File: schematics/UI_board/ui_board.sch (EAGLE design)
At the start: 116 parts, among them IC10 74HCT32N, IC11 74HCT14N, IC12 74HCT14N, IC13 74HCT393N, IC2 74HCT151N, IC3 74HCT32N, IC4 74HCT74N, IC5 74HCT08N, IC6 74HCT32N, IC7 74HCT14N, IC8 74HCT373N, IC9 74HCT32N

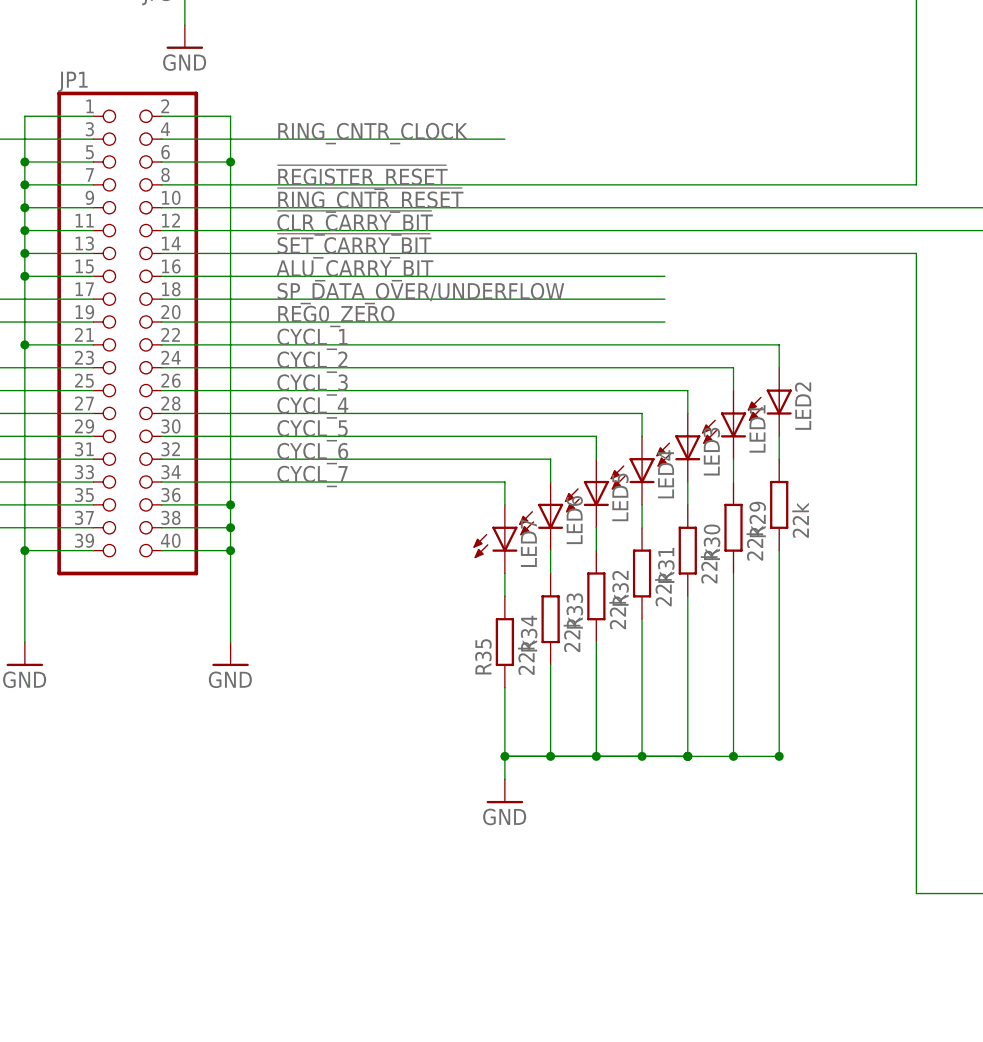
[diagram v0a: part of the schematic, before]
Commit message: feature freeze. I will now solder the Control Unit
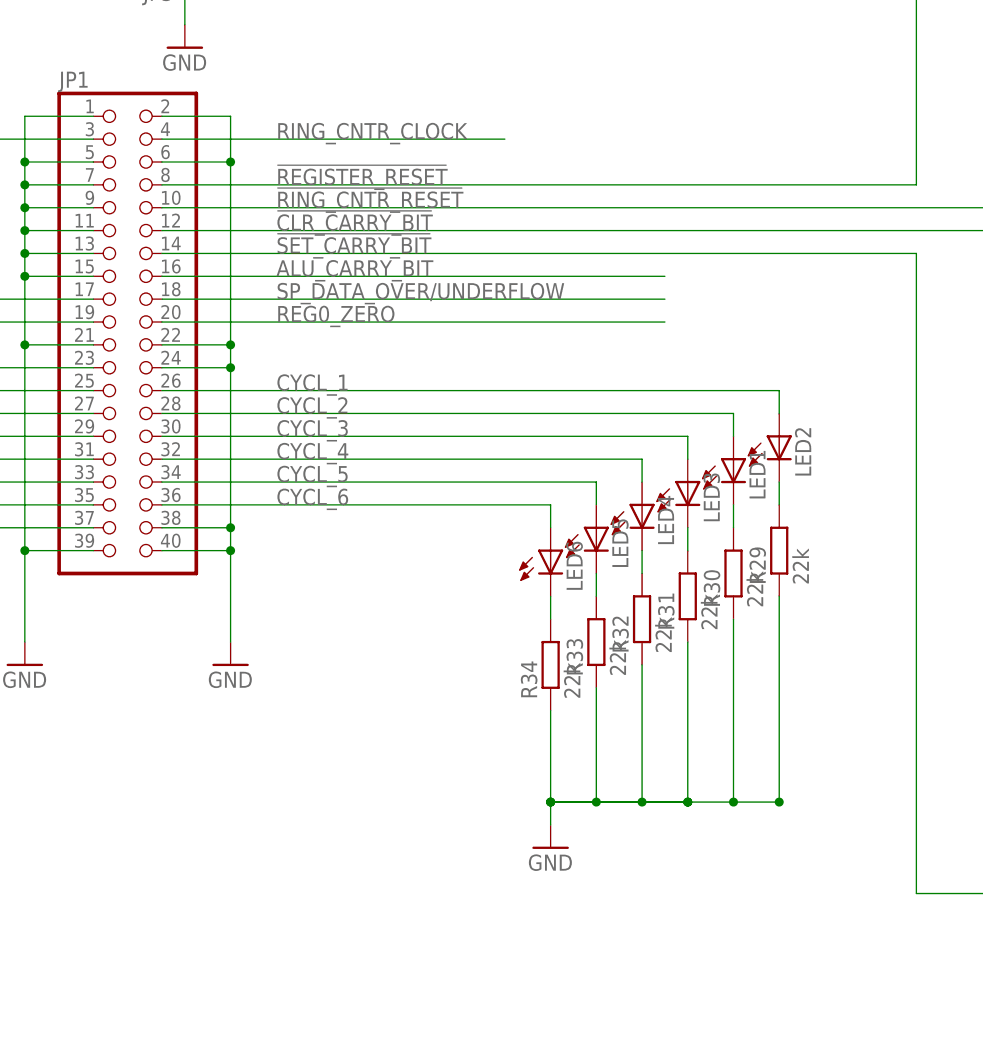
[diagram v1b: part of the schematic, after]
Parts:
- removed LED7: (no value), led:LED3MM
- removed R35: 22k, rcl:R-EU_R1206
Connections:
- removed net CYCL_7: JP1.34, LED7.A
- removed net N$66: LED7.C, R35.2
- net CYCL_1: now also JP1.26; no longer JP1.22
- net CYCL_2: now also JP1.28; no longer JP1.24
- net CYCL_3: now also JP1.30; no longer JP1.26
- net CYCL_4: now also JP1.32; no longer JP1.28
- net CYCL_5: now also JP1.34; no longer JP1.30
- net CYCL_6: now also JP1.36; no longer JP1.32
- net GND: now also JP1.22, JP1.24; no longer JP1.36, R35.1
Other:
- moved on the sheet: LED1, LED2, LED3, LED4, LED5, LED6, R29, R30, R31, R32, R33, R34
